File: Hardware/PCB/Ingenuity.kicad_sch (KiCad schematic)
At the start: 45 parts, among them J1 Conn_ST_STDC14, J2 Conn_02x20_Odd_Even, J3 Conn_02x05_Odd_Even, J4 Conn_01x02, J5 Conn_01x02, J7 Conn_01x03, J8 Conn_01x03, J9 Conn_01x02, Q1 NMOS, Q2 NMOS, SW1 SW_SPDT, SW101 SW_Push, U1 STM32L412KBTx, U3 LSM6DSM, U4 AMS1117-3.3

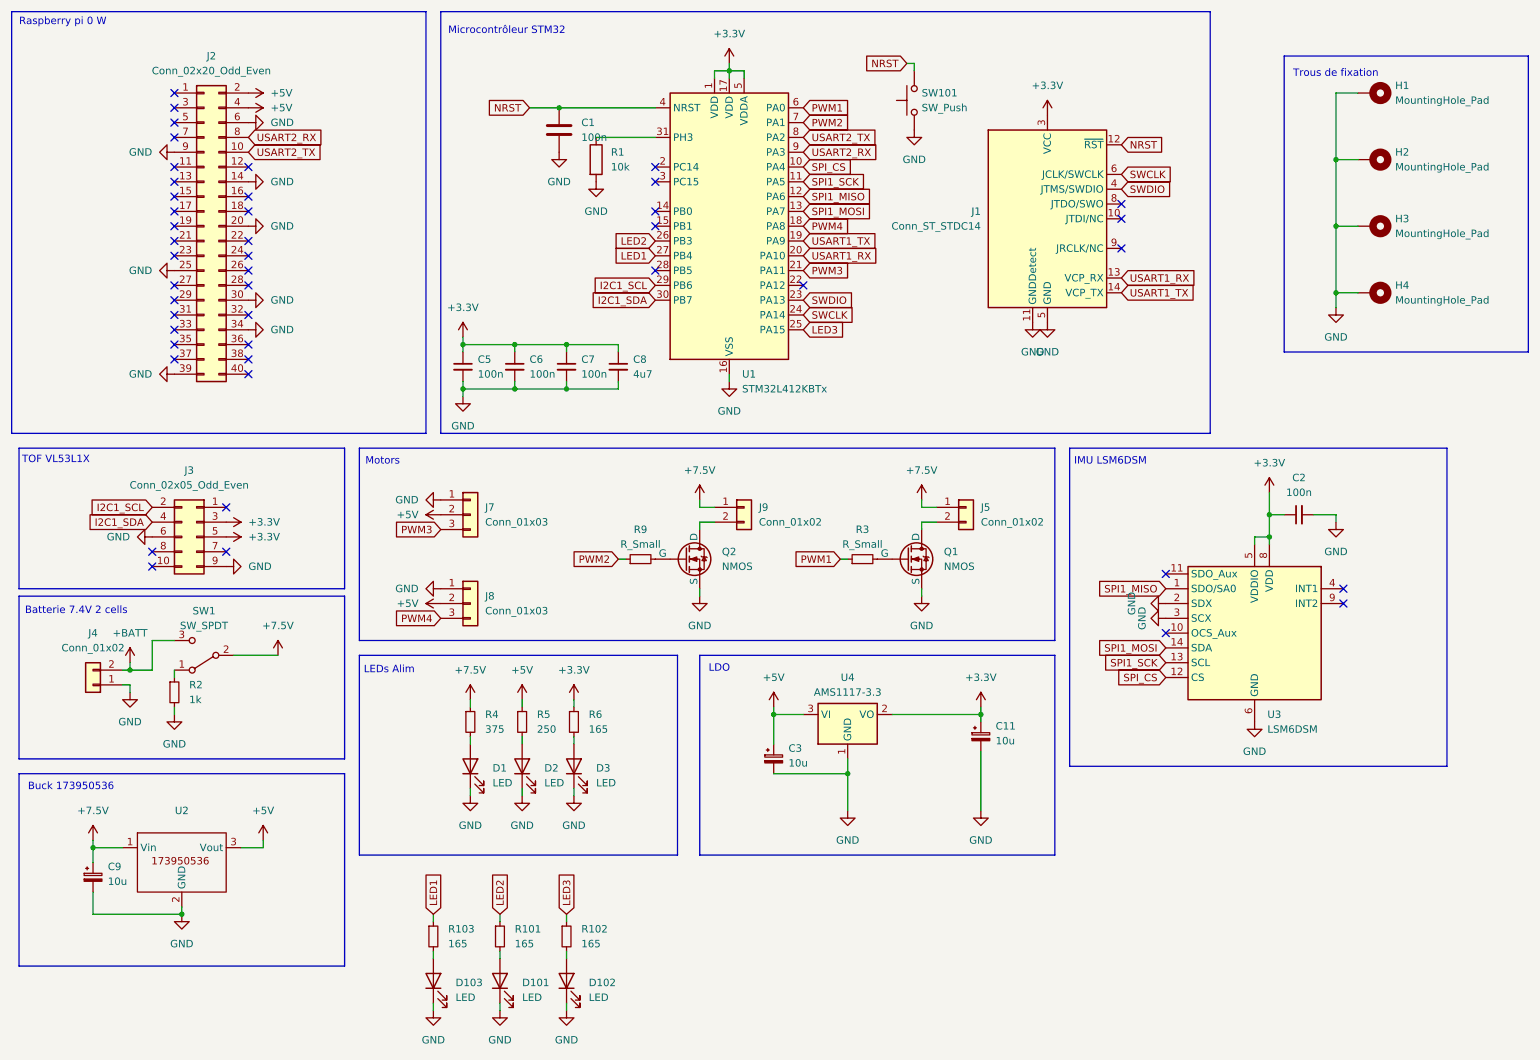
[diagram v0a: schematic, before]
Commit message: finalize pcb
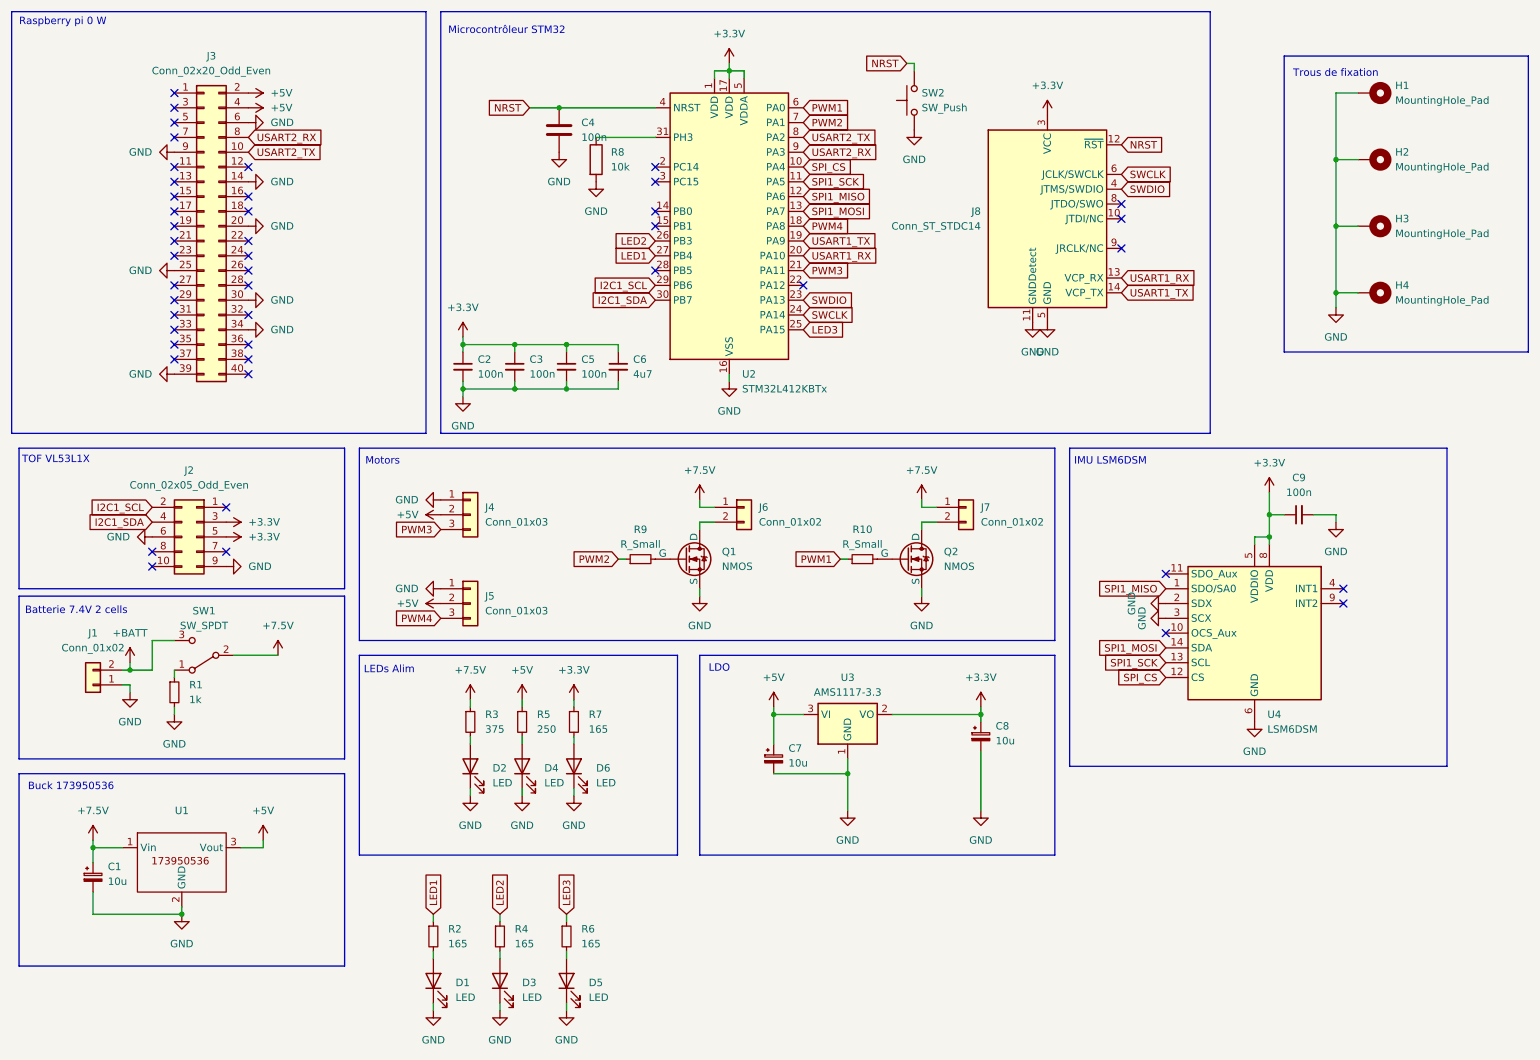
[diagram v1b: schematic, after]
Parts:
- renumbered C9 to C1, C5 to C2, C6 to C3, C1 to C4, C7 to C5, C8 to C6, C3 to C7, C11 to C8, C2 to C9, D103 to D1, D1 to D2, D101 to D3, D2 to D4, D102 to D5, D3 to D6, J4 to J1, J3 to J2, J2 to J3, J7 to J4, J8 to J5, J9 to J6, J5 to J7, J1 to J8, Q2 to Q1, Q1 to Q2, R2 to R1, R3 to R10, R103 to R2, R4 to R3, R101 to R4, R102 to R6, R6 to R7, R1 to R8, SW101 to SW2, U2 to U1, U1 to U2, U4 to U3, U3 to U4
